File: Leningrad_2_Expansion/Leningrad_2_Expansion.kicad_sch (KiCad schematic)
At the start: 2 parts, among them J1 ZX_Spectrum_Connector_48K, X6 Leningrad 2 Expansion Bus

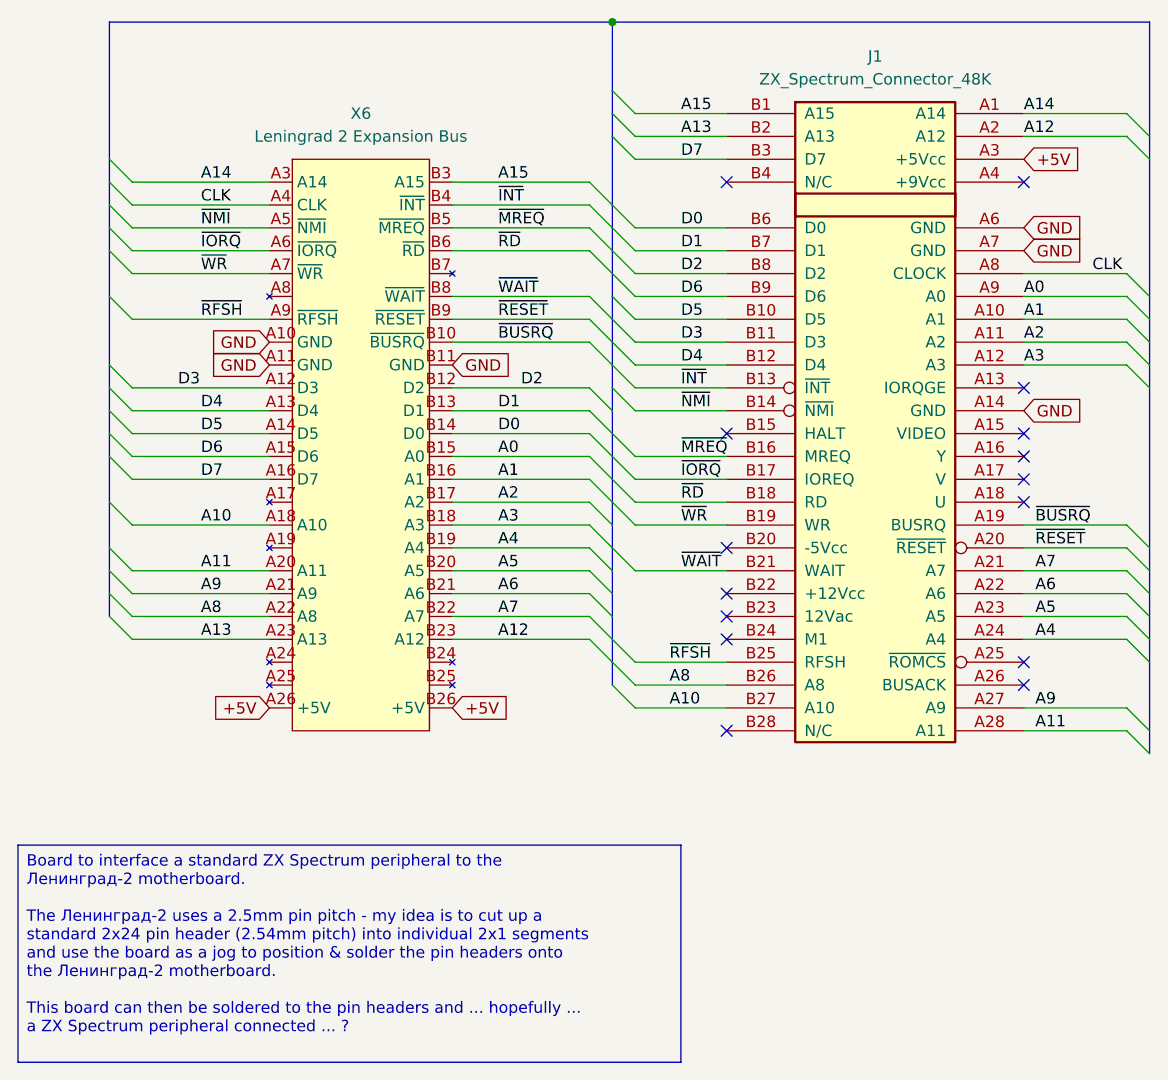
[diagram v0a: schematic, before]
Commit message: Updated Leningrad-2 symbol
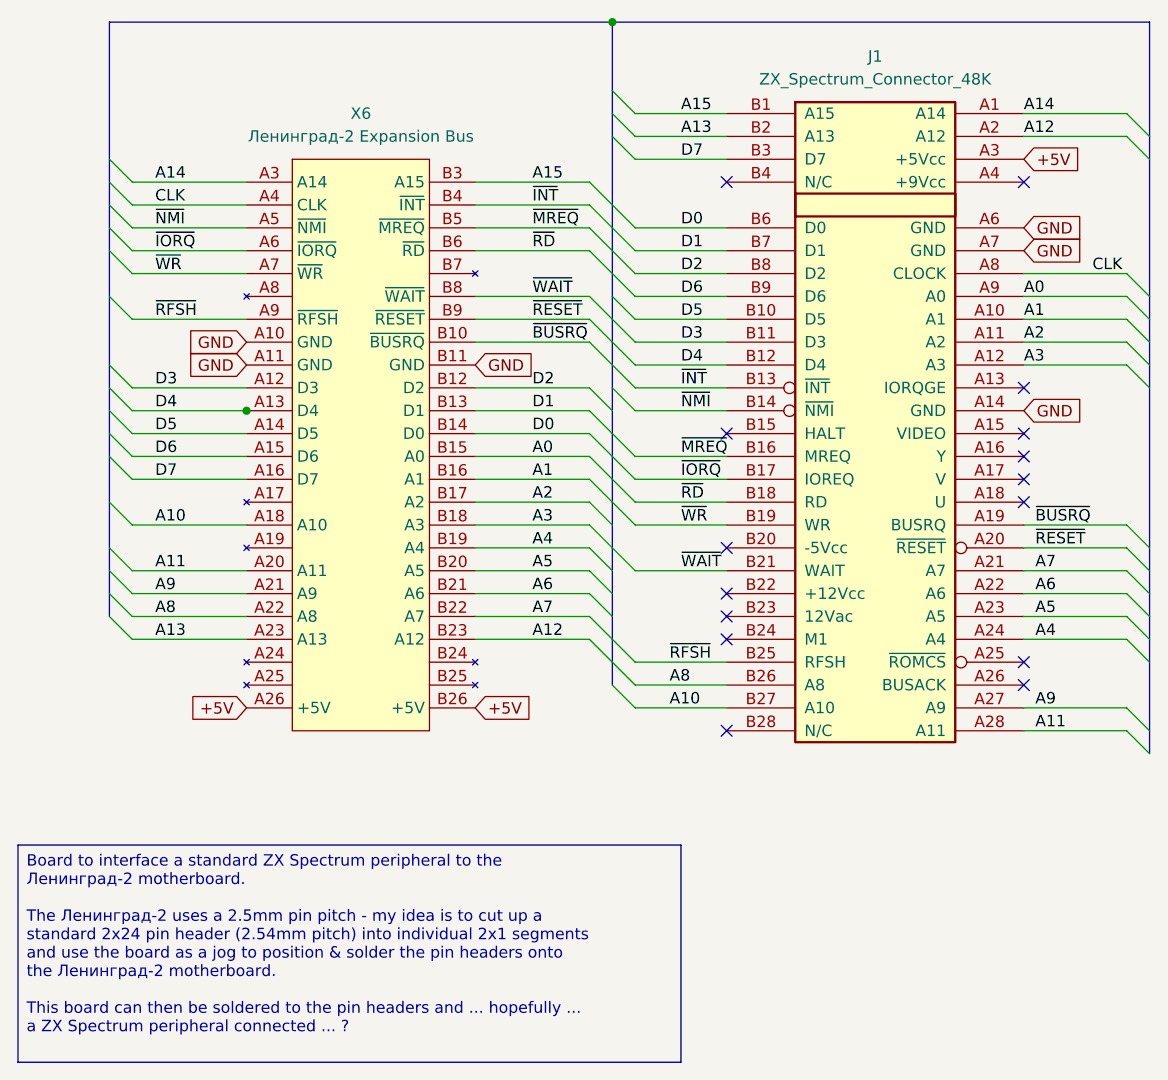
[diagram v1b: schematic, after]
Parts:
- X6: value Leningrad 2 Expansion Bus -> Ленинград-2 Expansion Bus
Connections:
- net D5: no longer X6.A14 (D5)
- net D6: no longer X6.A15 (D6)
- net D7: no longer X6.A16 (D7)
